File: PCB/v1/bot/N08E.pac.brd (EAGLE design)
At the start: 34 x 32.1 mm, 2 parts, among them J1 SMA-J-P-H-ST-EM1

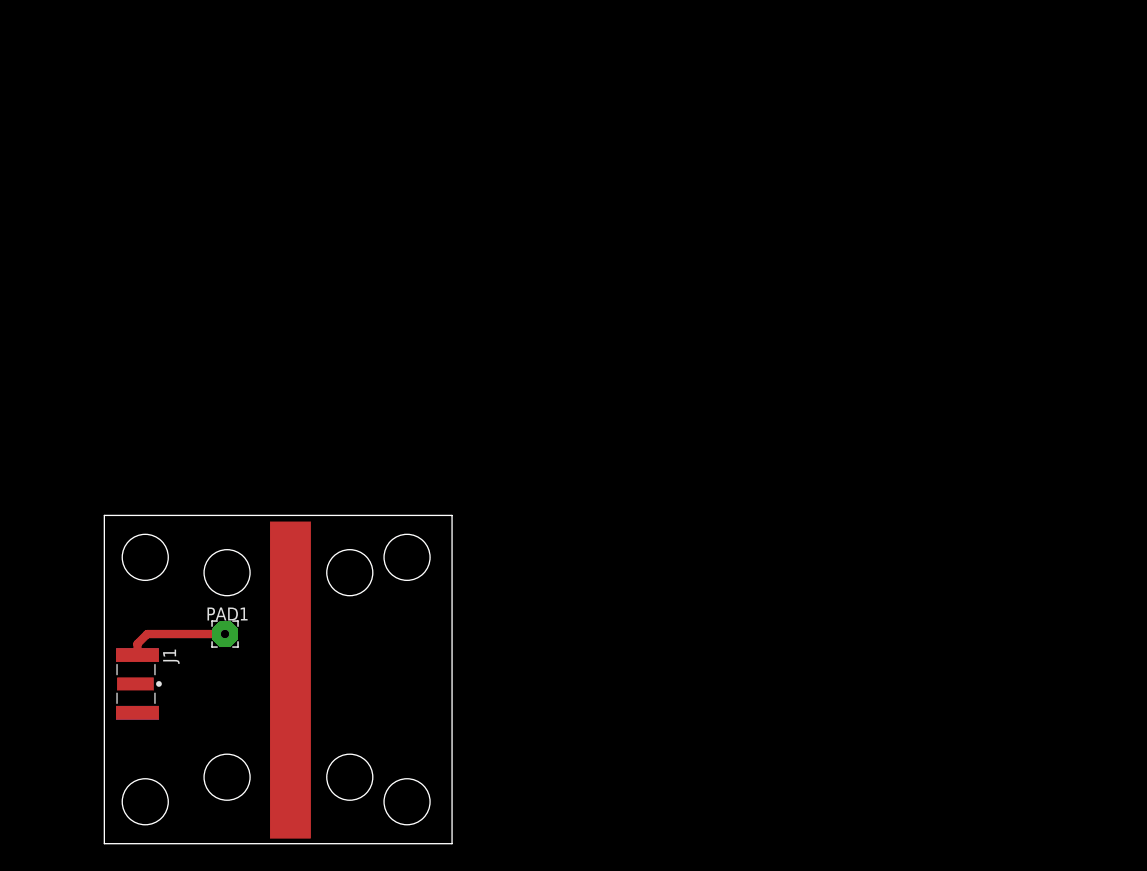
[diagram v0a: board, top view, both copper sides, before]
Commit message: updates
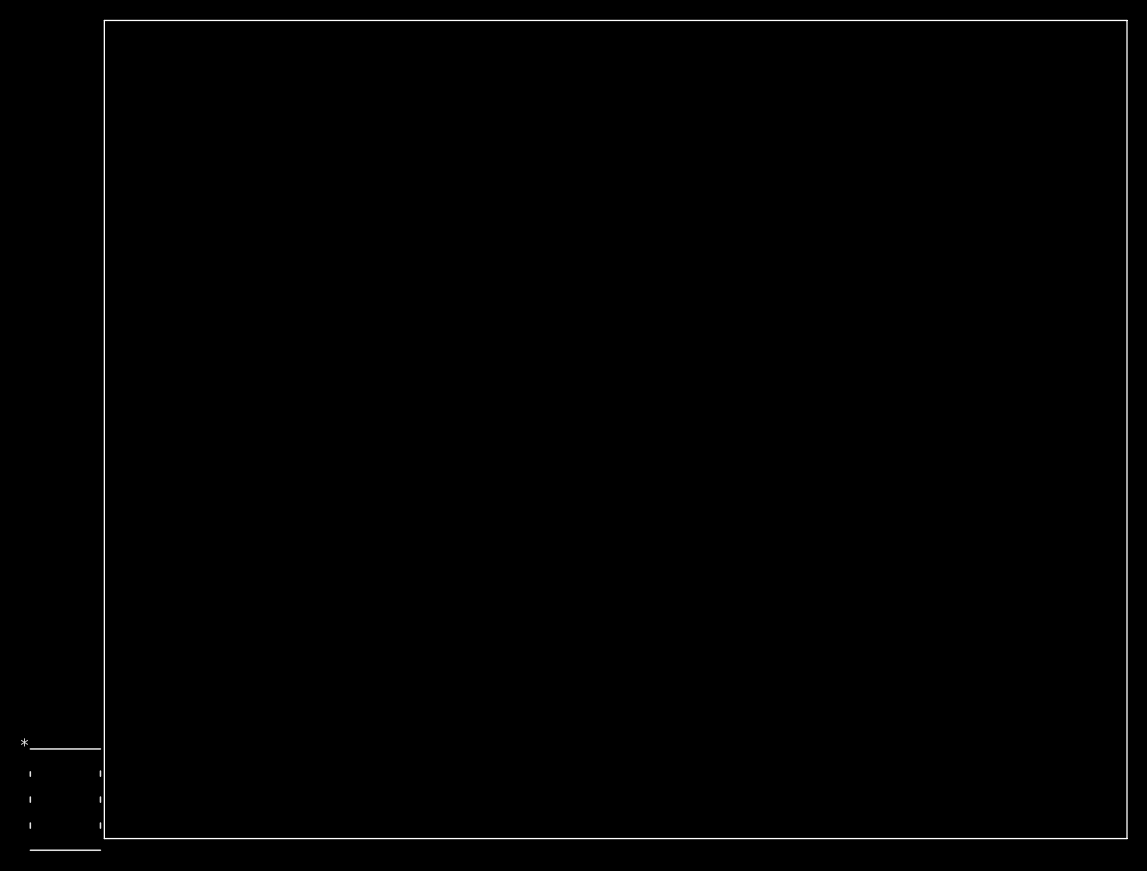
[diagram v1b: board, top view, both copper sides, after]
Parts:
- removed J1: SMA-J-P-H-ST-EM1, SMA-J-P-H-ST-EM1:SMA-J-P-H-ST-EM1
- removed PAD1: (no value), wirepad:2,54/0,8
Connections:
- removed net N$2: J1.2_1, J1.2_2, J1.3_1, J1.3_2, PAD1.1
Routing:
- net N$2: track 10.1 -> 0.00 mm
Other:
- board size 34 x 32.1 mm -> 100 x 80 mm
- board text added: "*"
- board text added: ">Name"
